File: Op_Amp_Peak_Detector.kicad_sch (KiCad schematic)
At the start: 12 parts, among them J1 Conn_01x03_Socket, J2 Conn_01x03_Socket, U1 OPA4340UA

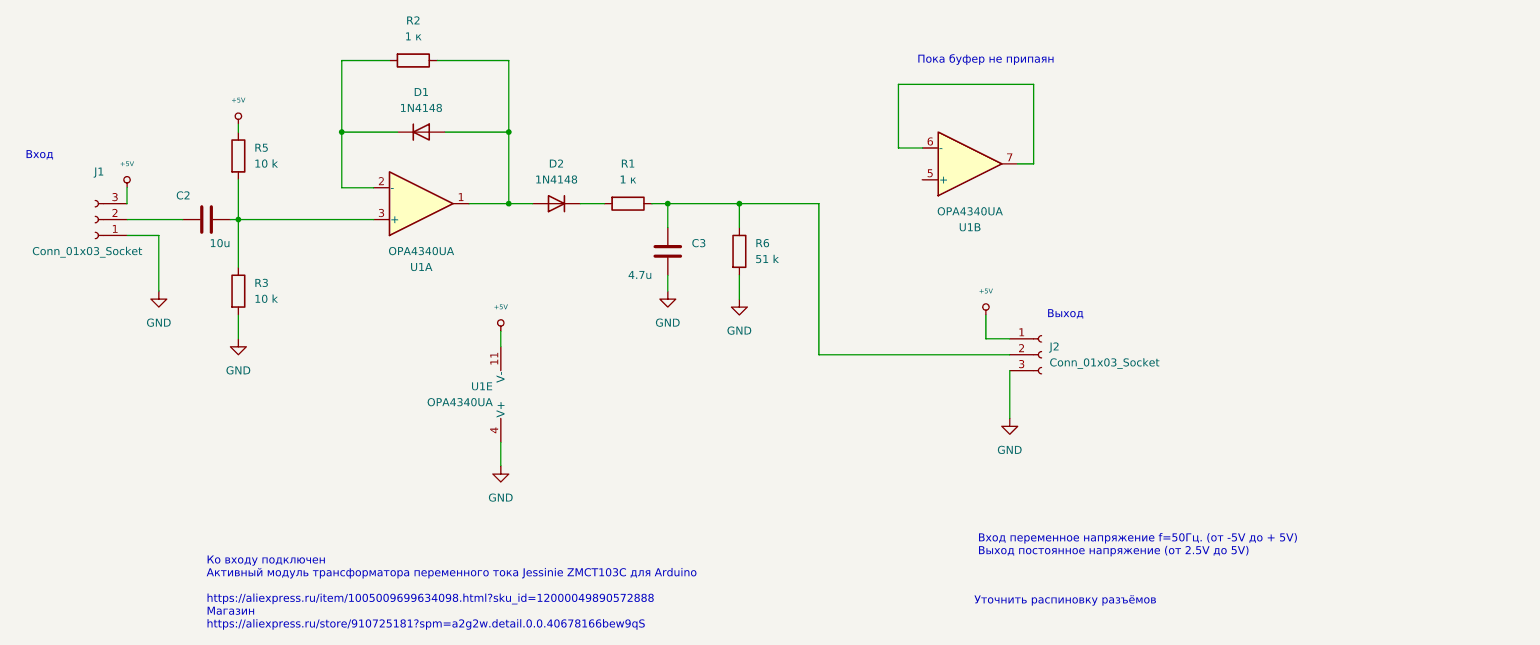
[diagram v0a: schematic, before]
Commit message: add buffer
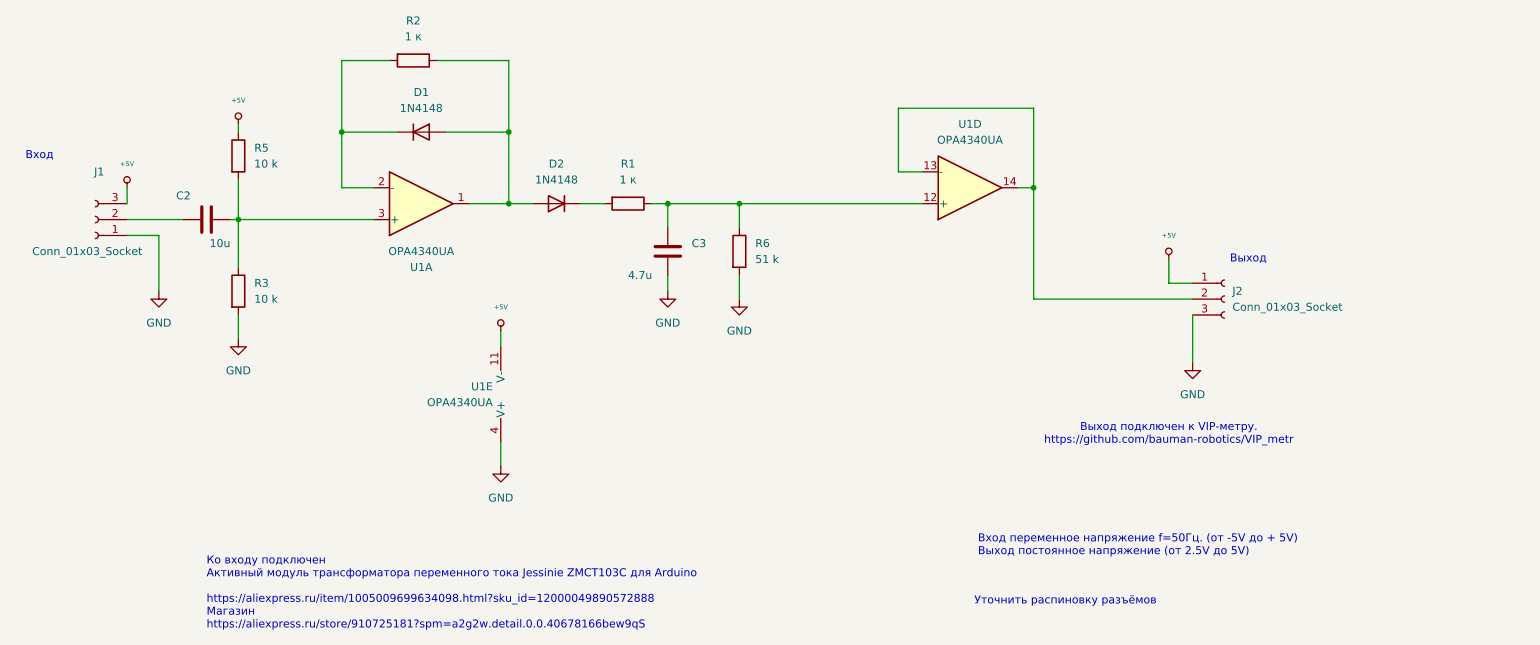
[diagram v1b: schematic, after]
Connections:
- net at C3.1, R1.1, R6.1: now also U1.12 (+); no longer J2.2 (Pin_2)
- new net: J2.2 (Pin_2), U1.13 (-), U1.14
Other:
- note added: "Выход подключен к VIP-метру. https://github.com/bauman-robotics/VIP_metr"
- note removed: "Пока буфер не припаян"
- moved on the sheet: J2, U1D
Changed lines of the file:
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@@
+	)
+	(junction
+		(at 200.66 49.53)
+		(diameter 0)
+		(color 0 0 0 0)
 	)
 	(junction
@@
 	(wire
 		(pts
-			(xy 196.85 76.2) (xy 166.37 76.2)
-		)
-		(stroke
-			(width 0)
-			(type default)
-		)
-	)
-	(wire
-		(pts
 			(xy 60.96 66.04) (xy 60.96 57.15)
 		)
@@
 	(wire
 		(pts
-			(xy 179.07 43.18) (xy 179.07 33.02)
+			(xy 179.07 46.99) (xy 179.07 36.83)
 		)
 		(stroke
@@
 	(wire
 		(pts
-			(xy 196.85 86.36) (xy 196.85 78.74)
+			(xy 226.06 77.47) (xy 226.06 69.85)
 		)
 		(stroke
@@
 	(wire
 		(pts
-			(xy 200.66 33.02) (xy 200.66 45.72)
-		)
-		(stroke
-			(width 0)
-			(type default)
-		)
-	)
-	(wire
-		(pts
-			(xy 196.85 73.66) (xy 193.04 73.66)
-		)
-		(stroke
-			(width 0)
-			(type default)
-		)
-	)
-	(wire
-		(pts
-			(xy 179.07 33.02) (xy 200.66 33.02)
+			(xy 226.06 64.77) (xy 222.25 64.77)
+		)
+		(stroke
+			(width 0)
+			(type default)
+		)
+	)
+	(wire
+		(pts
+			(xy 179.07 36.83) (xy 200.66 36.83)
 		)
 		(stroke
@@
 	(wire
 		(pts
-			(xy 166.37 76.2) (xy 166.37 52.07)
-		)
-		(stroke
-			(width 0)
-			(type default)
-		)
-	)
-	(wire
-		(pts
 			(xy 110.49 52.07) (xy 116.84 52.07)
 		)
@@
 	(wire
 		(pts
+			(xy 200.66 67.31) (xy 200.66 49.53)
+		)
+		(stroke
+			(width 0)
+			(type default)
+		)
+	)
+	(wire
+		(pts
+			(xy 226.06 67.31) (xy 200.66 67.31)
+		)
+		(stroke
+			(width 0)
+			(type default)
+		)
+	)
+	(wire
+		(pts
 			(xy 90.17 29.21) (xy 90.17 40.64)
 		)
@@
 	(wire
 		(pts
-			(xy 193.04 73.66) (xy 193.04 69.85)
-		)
-		(stroke
-			(width 0)
-			(type default)
-		)
-	)
-	(wire
-		(pts
-			(xy 153.67 52.07) (xy 166.37 52.07)
+			(xy 222.25 64.77) (xy 222.25 60.96)
+		)
+		(stroke
+			(width 0)
+			(type default)
+		)
+	)
+	(wire
+		(pts
+			(xy 153.67 52.07) (xy 182.88 52.07)
 		)
 		(stroke
@@
 	(wire
 		(pts
-			(xy 182.88 43.18) (xy 179.07 43.18)
+			(xy 182.88 46.99) (xy 179.07 46.99)
 		)
 		(stroke
@@
 	(wire
 		(pts
-			(xy 200.66 45.72) (xy 198.12 45.72)
+			(xy 200.66 49.53) (xy 198.12 49.53)
 		)
 		(stroke
@@
 	(wire
 		(pts
+			(xy 200.66 36.83) (xy 200.66 49.53)
+		)
+		(stroke
+			(width 0)
+			(type default)
+		)
+	)
+	(wire
+		(pts
 			(xy 153.67 55.88) (xy 153.67 52.07)
 		)
@@
 		)
 	)
-	(text "Пока буфер не припаян"
-		(exclude_from_sim no)
-		(at 193.04 29.21 0)
+	(text "Выход подключен к VIP-метру. \nhttps://github.com/bauman-robotics/VIP_metr"
+		(exclude_from_sim no)
+		(at 222.25 88.9 0)
 		(effects
 			(font
@@
 	(text "Выход"
 		(exclude_from_sim no)
-		(at 205.74 69.85 0)
+		(at 234.95 60.96 0)
 		(effects
 			(font
@@
 	(symbol
 		(lib_id "Connector:Conn_01x03_Socket")
-		(at 201.93 76.2 0)
+		(at 231.14 67.31 0)
 		(unit 1)
 		(exclude_from_sim no)
@@
 		(fields_autoplaced yes)
 		(property "Reference" "J2"
-			(at 203.2 74.9299 0)
+			(at 232.41 66.0399 0)
 			(effects
 				(font
@@
 		)
 		(property "Value" "Conn_01x03_Socket"
-			(at 203.2 77.4699 0)
+			(at 232.41 68.5799 0)
 			(effects
 				(font
@@
 		)
 		(property "Footprint" ""
-			(at 201.93 76.2 0)
+			(at 231.14 67.31 0)
 			(effects
 				(font
@@
 		)
 		(property "Datasheet" "~"
-			(at 201.93 76.2 0)
+			(at 231.14 67.31 0)
 			(effects
 				(font
@@
 		)
 		(property "Description" "Generic connector, single row, 01x03, script generated"
-			(at 201.93 76.2 0)
+			(at 231.14 67.31 0)
 			(effects
 				(font
@@
 	(symbol
 		(lib_id "power:GND")
-		(at 196.85 86.36 0)
+		(at 226.06 77.47 0)
 		(unit 1)
 		(exclude_from_sim no)
@@
 		(fields_autoplaced yes)
 		(property "Reference" "#PWR6"
-			(at 196.85 92.71 0)
+			(at 226.06 83.82 0)
 			(effects
 				(font
@@
 		)
 		(property "Value" "GND"
-			(at 196.85 91.44 0)
+			(at 226.06 82.55 0)
 			(effects
 				(font
@@
 		)
 		(property "Footprint" ""
-			(at 196.85 86.36 0)
+			(at 226.06 77.47 0)
 			(effects
 				(font
@@
 		)
 		(property "Datasheet" ""
-			(at 196.85 86.36 0)
+			(at 226.06 77.47 0)
 			(effects
 				(font
@@
 		)
 		(property "Description" "Power symbol creates a global label with name \"GND\" , ground"
-			(at 196.85 86.36 0)
+			(at 226.06 77.47 0)
 			(effects
 				(font
@@
 	(symbol
 		(lib_id "Bpi_v3_Lib:VCC")
-		(at 193.04 69.85 0)
+		(at 222.25 60.96 0)
 		(unit 1)
 		(exclude_from_sim no)
@@
 		(fields_autoplaced yes)
 		(property "Reference" "#PWR3"
-			(at 193.04 67.31 0)
+			(at 222.25 58.42 0)
 			(effects
 				(font
@@
 		)
 		(property "Value" "+5V"
-			(at 193.04 66.04 0)
+			(at 222.25 57.15 0)
 			(effects
 				(font
@@
 		)
 		(property "Footprint" ""
-			(at 193.04 69.85 0)
+			(at 222.25 60.96 0)
 			(effects
 				(font
@@
 		)
 		(property "Datasheet" ""
-			(at 193.04 69.85 0)
+			(at 222.25 60.96 0)
 			(effects
 				(font
@@
 		)
 		(property "Description" ""
-			(at 193.04 69.85 0)
+			(at 222.25 60.96 0)
 			(effects
 				(font
@@
 	(symbol
 		(lib_id "Amplifier_Operational:OPA4340UA")
-		(at 190.5 45.72 0)
+		(at 190.5 49.53 0)
 		(mirror x)
-		(unit 2)
+		(unit 4)
 		(exclude_from_sim no)
 		(in_bom yes)
@@
 		(fields_autoplaced yes)
 		(property "Reference" "U1"
-			(at 190.5 55.88 0)
+			(at 190.5 39.37 0)
 			(effects
 				(font
@@
 		)
 		(property "Value" "OPA4340UA"
-			(at 190.5 53.34 0)
+			(at 190.5 41.91 0)
 			(effects
 				(font
@@
 		)
 		(property "Footprint" ""
-			(at 189.23 48.26 0)
+			(at 189.23 52.07 0)
 			(effects
 				(font
@@
 		)
 		(property "Datasheet" "http://www.ti.com/lit/ds/symlink/opa340.pdf"
-			(at 191.77 50.8 0)
+			(at 191.77 54.61 0)
 			(effects
 				(font
@@
 		)
 		(property "Description" "Quad Single-Supply, Rail-to-Rail Operational Amplifier, MicroAmplifier Series, SOIC-14"
-			(at 190.5 45.72 0)
+			(at 190.5 49.53 0)
 			(effects
 				(font
@@
 				(path "/268cd6af-7866-4698-8209-c82979dea447"
 					(reference "U1")
-					(unit 2)
-				)
-			)
+					(unit 4)
+				)
+			)
